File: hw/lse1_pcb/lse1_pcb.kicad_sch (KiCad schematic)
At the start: 49 parts, among them M1 Motor_3pin, Q1 IRFR1205, Q2 IRFR1205, Q3 IRFR1205, Q4 IRFR1205, Q5 IRFR1205, Q6 IRFR1205, U1 IR2301, U2 IR2301, U3 IR2301, U4 AZ1084CD-5.0TRG1, U5 LM339, U6 EK-TM4C123GXL

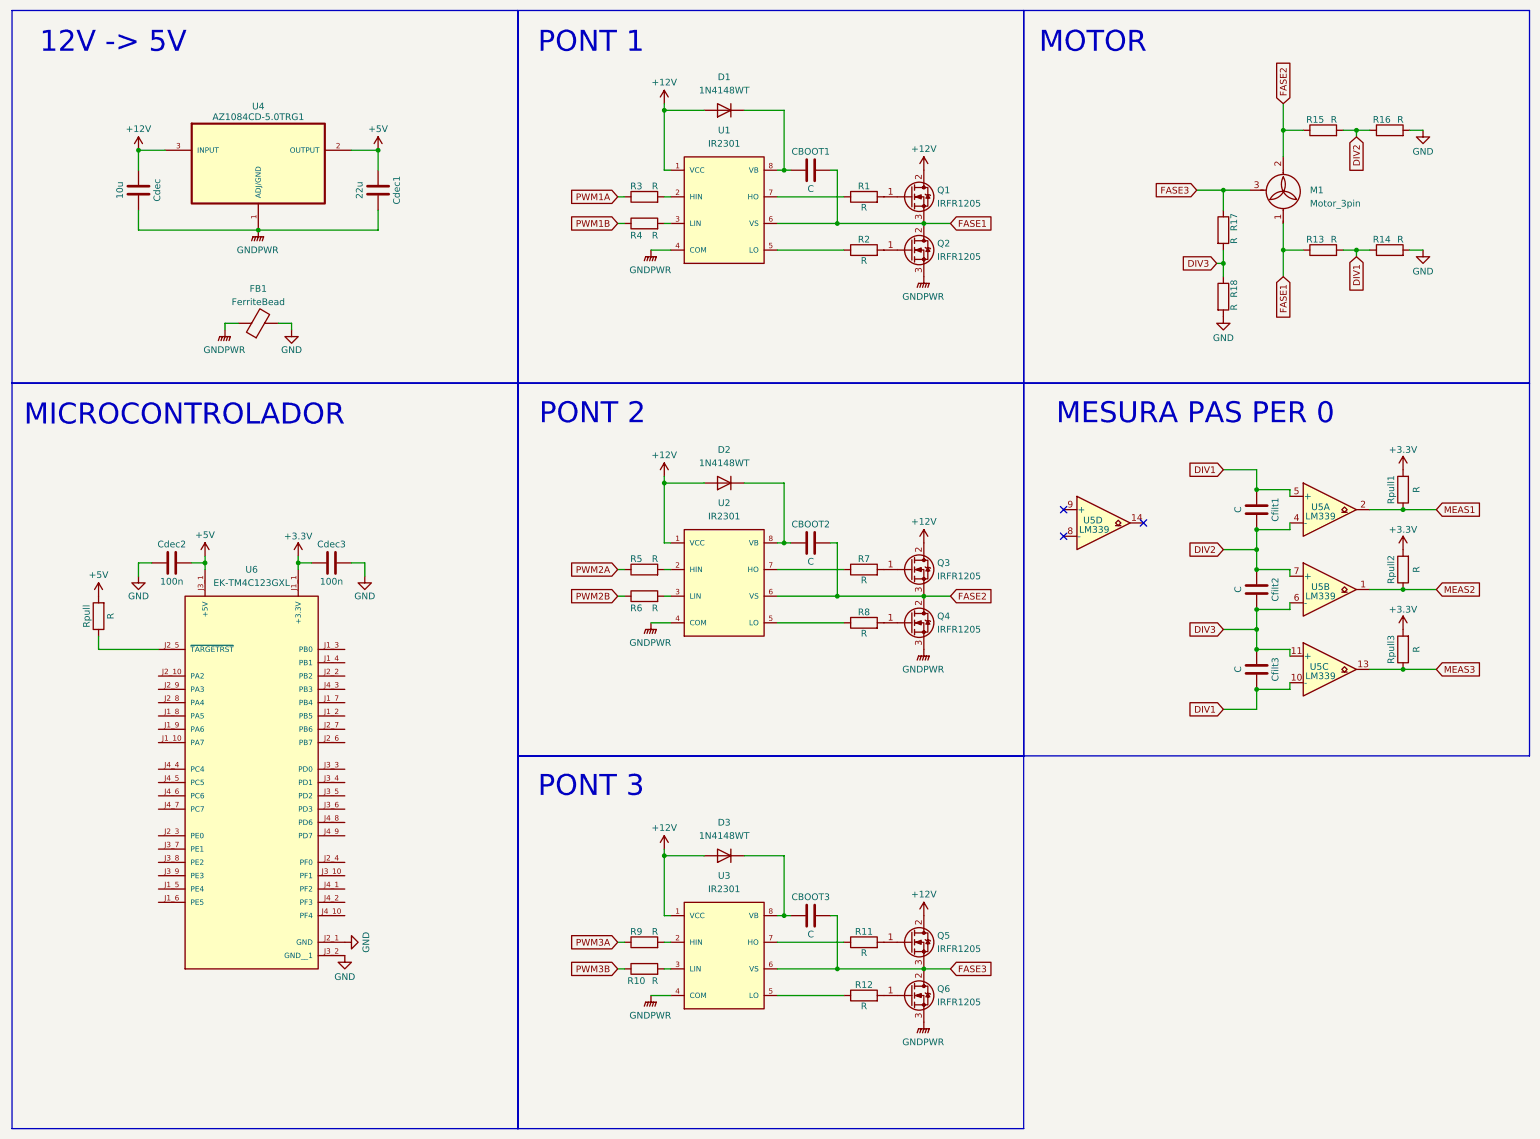
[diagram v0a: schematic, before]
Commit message: schem done
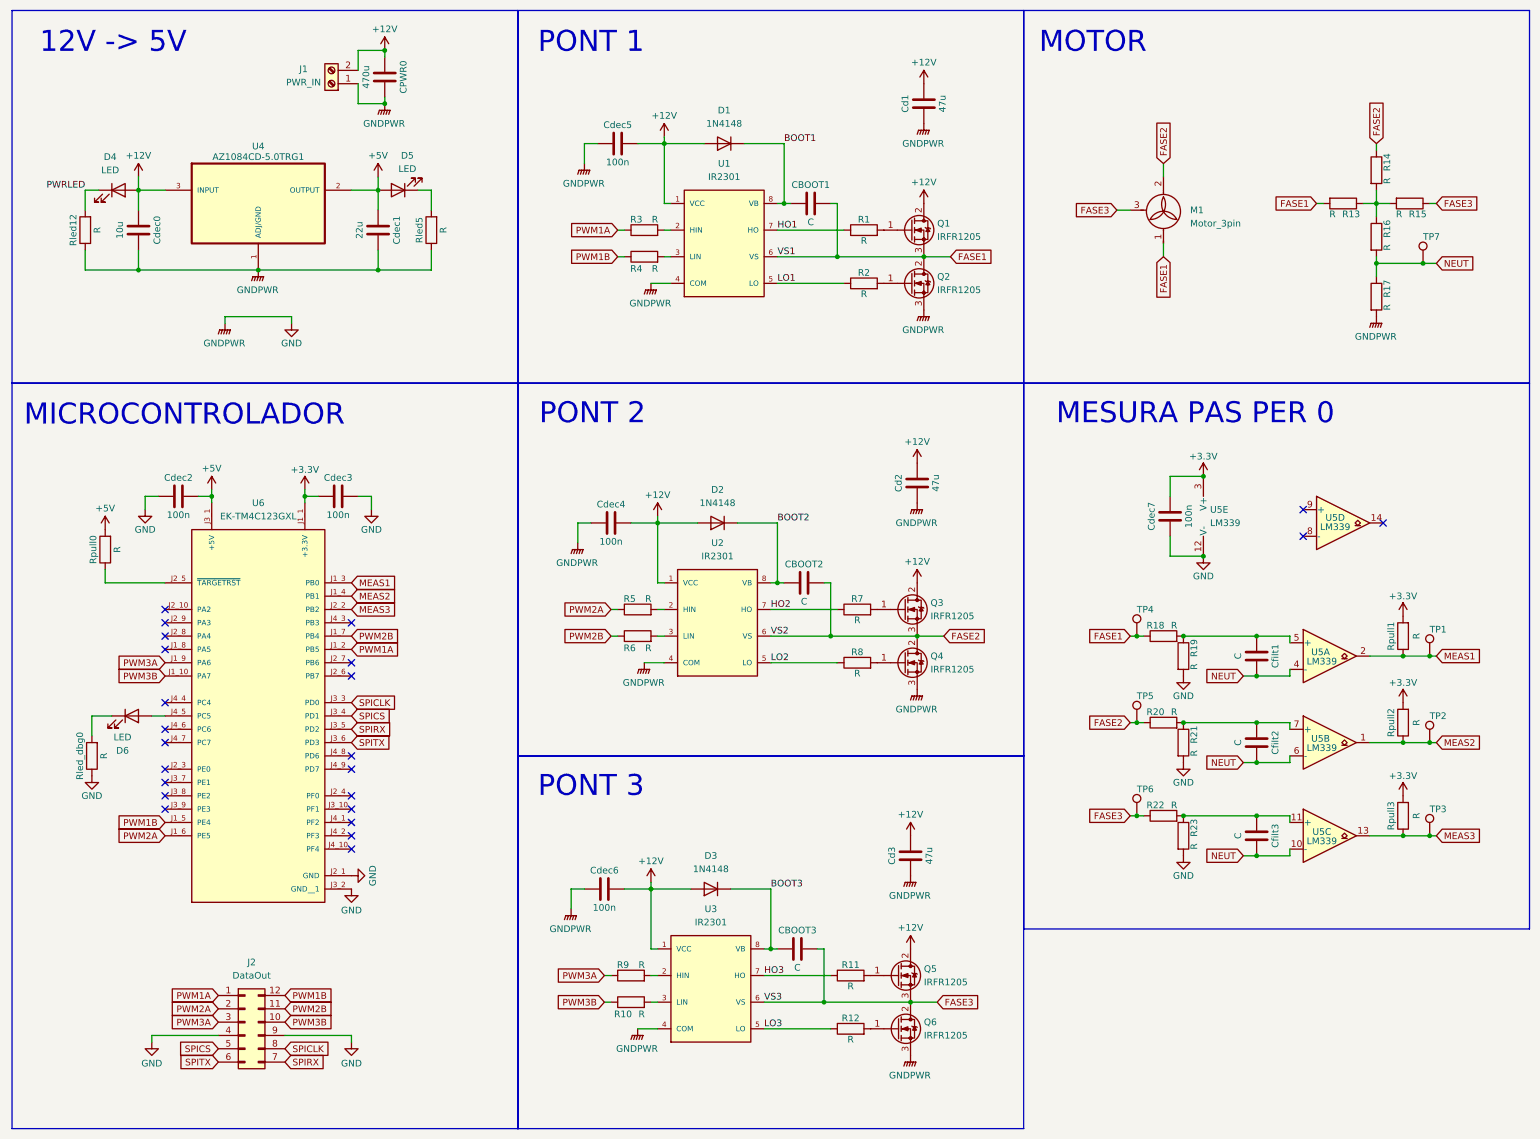
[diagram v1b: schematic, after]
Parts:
- removed D1, D2, D3: 1N4148WT, Diode_SMD:D_SOD-523, symbol Diode:1N4148WT
- removed FB1: FerriteBead, symbol Device:FerriteBead
- added CPWR0: 470u, Capacitor_SMD:C_Elec_10x10.2, symbol Device:C
- added Cd1, Cd2, Cd3: 47u, Capacitor_SMD:C_1206_3216Metric, symbol Device:C
- added Cdec4, Cdec5, Cdec6, Cdec7: 100n, Capacitor_SMD:C_1206_3216Metric, symbol Device:C
- added D1, D2, D3: 1N4148, Diode_THT:D_DO-35_SOD27_P7.62mm_Horizontal, symbol Diode:1N4148
- added D4, D5, D6: LED, LED_SMD:LED_0805_2012Metric, symbol Device:LED
- added J1: PWR_IN, Connector_Samtec_HPM_THT:Samtec_HPM-02-01-x-S_Straight_1x02_Pitch5.08mm, symbol Connector:Screw_Terminal_01x02
- added J2: DataOut, Connector_PinHeader_2.54mm:PinHeader_2x06_P2.54mm_Vertical, symbol Connector_Generic:Conn_02x06_Counter_Clockwise
- added R19, R20, R21, R22, R23, Rled12, Rled5, Rled_dbg0: R, Resistor_SMD:R_1206_3216Metric, symbol Device:R
- added TP1, TP2, TP3, TP4, TP5, TP6, TP7: TestPoint, Connector_PinHeader_2.54mm:PinHeader_1x01_P2.54mm_Vertical, symbol Connector:TestPoint
- added unit 5 of U5
- CBOOT1, CBOOT2, CBOOT3, Cdec1, Cdec2, Cdec3, Cfilt1, Cfilt2, Cfilt3: footprint (none) -> Capacitor_SMD:C_1206_3216Metric
- Cdec0: renamed from Cdec; footprint (none) -> Capacitor_SMD:C_1206_3216Metric
- M1: footprint (none) -> Connector_Samtec_HPM_THT:Samtec_HPM-03-01-x-S_Straight_1x03_Pitch5.08mm
- R1, R10, R11, R12, R13, R14, R15, R16, R17, R18, R2, R3, R4, R5, R6, R7, R8, R9, Rpull1, Rpull2, Rpull3: footprint (none) -> Resistor_SMD:R_1206_3216Metric
- Rpull0: renamed from Rpull; footprint (none) -> Resistor_SMD:R_1206_3216Metric
- U1, U2, U3: footprint (none) -> Package_SO:SOIC-8_3.9x4.9mm_P1.27mm
- U5: footprint (none) -> Package_SO:SOIC-14_3.9x8.7mm_P1.27mm
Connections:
- net GNDPWR is gone; now on net GND: Cdec0.2, Cdec1.2, Q2.3 (S), Q4.3 (S), Q6.3 (S), U1.4 (COM), U2.4 (COM), U3.4 (COM), U4.1 (ADJ/GND)
- net +12V: now also CPWR0.1, Cd1.2, Cd2.2, Cd3.2, Cdec4.2, Cdec5.2, Cdec6.2, D1.2 (A), D2.2 (A), D3.2 (A), D4.2 (A), J1.2 (Pin_2)
- net +3.3V: now also Cdec7.2, U5.3 (V+)
- net +5V: now also D5.2 (A)
- net FASE1: now also R13.2, R18.1, TP4.1; no longer R13.1
- net FASE2: now also R14.1, R20.1, TP5.1; no longer R15.1
- net FASE3: now also R15.1, R22.1, TP6.1; no longer R17.1
- net GND: now also R17.2, CPWR0.2, Cd1.1, Cd2.1, Cd3.1, Cdec4.1, Cdec5.1, Cdec6.1, Cdec7.1, J1.1 (Pin_1), J2.4 (Pin_4), J2.9 (Pin_9), R19.2, R21.2, R23.2, Rled12.1, Rled5.1, Rled_dbg0.1, U5.12 (V-); no longer R14.2, R16.2, R18.2
- net MEAS1: now also U6.J1_3 (PB0), TP1.1
- net MEAS2: now also U6.J1_4 (PB1), TP2.1
- net MEAS3: now also U6.J2_2 (PB2), TP3.1
- net PWM1A: now also U6.J1_2 (PB5), J2.1 (Pin_1)
- net PWM1B: now also U6.J1_5 (PE4), J2.12 (Pin_12)
- net PWM2A: now also U6.J1_6 (PE5), J2.2 (Pin_2)
- net PWM2B: now also U6.J1_7 (PB4), J2.11 (Pin_11)
- net PWM3A: now also U6.J1_9 (PA6), J2.3 (Pin_3)
- net PWM3B: now also U6.J1_10 (PA7), J2.10 (Pin_10)
- net LO1: now reaches R2.1, U1.5 (LO)
- net HO1: now reaches R1.1, U1.7 (HO)
- net BOOT1: now reaches CBOOT1.1, U1.8 (VB)
- net BOOT1: now also D1.1 (K)
- net LO2: now reaches R8.1, U2.5 (LO)
- net BOOT2: now reaches CBOOT2.1, U2.8 (VB)
- net BOOT2: now also D2.1 (K)
- net SPICLK: now reaches U6.J3_3 (PD0)
- net SPICLK: now also J2.8 (Pin_8)
- net SPICS: now reaches U6.J3_4 (PD1)
- net SPICS: now also J2.5 (Pin_5)
- net SPIRX: now reaches U6.J3_5 (PD2)
- net SPIRX: now also J2.7 (Pin_7)
- net SPITX: now reaches U6.J3_6 (PD3)
- net SPITX: now also J2.6 (Pin_6)
- net at U6.J4_5 (PC5): now also D6.2 (A)
- net HO2: now reaches R7.1, U2.7 (HO)
- net HO3: now reaches R11.1, U3.7 (HO)
- net BOOT3: now reaches CBOOT3.1, U3.8 (VB)
- net BOOT3: now also D3.1 (K)
- net LO3: now reaches R12.1, U3.5 (LO)
- removed net DIV1: Cfilt1.1, Cfilt3.2, R13.2, R14.1, U5.10 (-), U5.5 (+)
- removed net DIV2: Cfilt1.2, Cfilt2.1, R15.2, R16.1, U5.4 (-), U5.7 (+)
- removed net DIV3: Cfilt2.2, Cfilt3.1, R17.2, R18.1, U5.11 (+), U5.6 (-)
- new net: Cfilt2.1, R20.2, R21.1, U5.7 (+)
- new net: Cfilt3.1, R22.2, R23.1, U5.11 (+)
- new net: Cfilt1.1, R18.2, R19.1, U5.5 (+)
- new net: D5.1 (K), Rled5.2
- new net: R13.1, R14.2, R15.2, R16.1
- new net: D6.1 (K), Rled_dbg0.2
- new net NEUT: Cfilt1.2, Cfilt2.2, Cfilt3.2, R16.2, R17.1, TP7.1, U5.10 (-), U5.4 (-), U5.6 (-)
- new net PWRLED: D4.1 (K), Rled12.2
- no-connect marks 3 -> 24
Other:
- company: (none) -> Adrià Brú & Miquel Limón
- title: (none) -> PCB LSE1 FIUUMMM
- moved on the sheet: CBOOT1, CBOOT2, CBOOT3, Cdec0, Cdec1, Cdec2, Cdec3, Cfilt1, Cfilt2, Cfilt3, M1, Q1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

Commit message: difference describe/commit?
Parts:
- U6: footprint EK-TM4C123GXL:MODULE_EK-TM4C123GXL -> models:MODULE_EK-TM4C123GXL
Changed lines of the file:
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@@
 			)
 		)
-		(property "Footprint" "EK-TM4C123GXL:MODULE_EK-TM4C123GXL"
+		(property "Footprint" "models:MODULE_EK-TM4C123GXL"
 			(at 59.69 144.78 0)
 			(effects

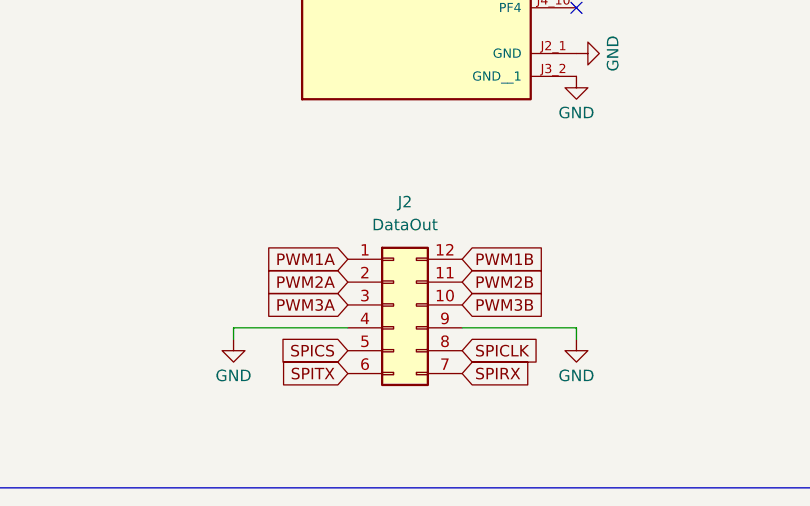
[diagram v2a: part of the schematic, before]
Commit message: ponts fets
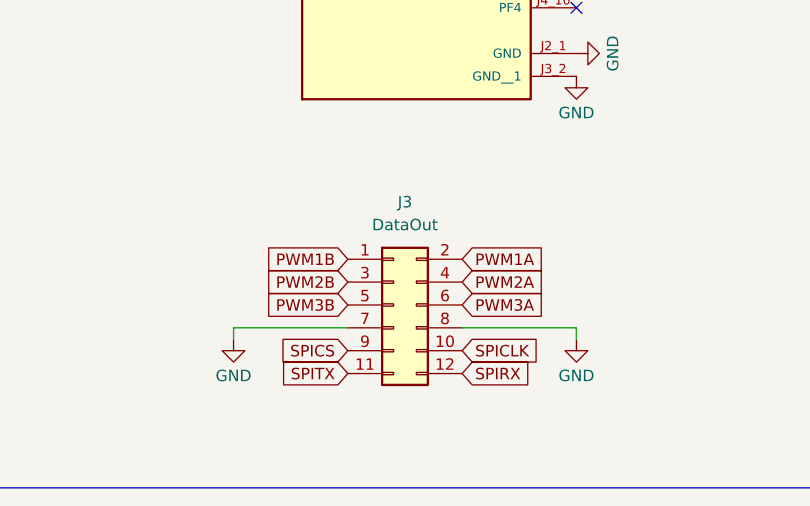
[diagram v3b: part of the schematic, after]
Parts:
- removed J2: DataOut, Connector_PinHeader_2.54mm:PinHeader_2x06_P2.54mm_Vertical, symbol Connector_Generic:Conn_02x06_Counter_Clockwise
- added J3: DataOut, Connector_PinHeader_2.54mm:PinHeader_2x06_P2.54mm_Vertical, symbol Connector_Generic:Conn_02x06_Odd_Even
- U4: footprint AZ1084CD-5.0TRG1:DPAK457P1010X238-3N -> models_cachy:DPAK457P1010X238-3N
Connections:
- net GND: now also J3.7 (Pin_7), J3.8 (Pin_8)
- net PWM1A: now also J3.2 (Pin_2)
- net PWM1B: now also J3.1 (Pin_1)
- net PWM2A: now also J3.4 (Pin_4)
- net PWM2B: now also J3.3 (Pin_3)
- net PWM3A: now also J3.6 (Pin_6)
- net PWM3B: now also J3.5 (Pin_5)
- net SPICLK: now also J3.10 (Pin_10)
- net SPICS: now also J3.9 (Pin_9)
- net SPIRX: now also J3.12 (Pin_12)
- net SPITX: now also J3.11 (Pin_11)
